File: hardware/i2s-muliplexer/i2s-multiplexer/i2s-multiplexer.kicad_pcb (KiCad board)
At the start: 2 copper layers, 64.5 x 63.5 mm, 35 parts, among them J1 Conn_01x05, J2 Conn_01x05, J3 Conn_01x05, J4 Conn_01x05, J5 Conn_01x05, J6 Conn_01x05, J7 Conn_01x07, J8 Conn_01x05, U1 74HC244, U2 74HC244, U3 74HC244, U4 74HC126, U5 74LS138

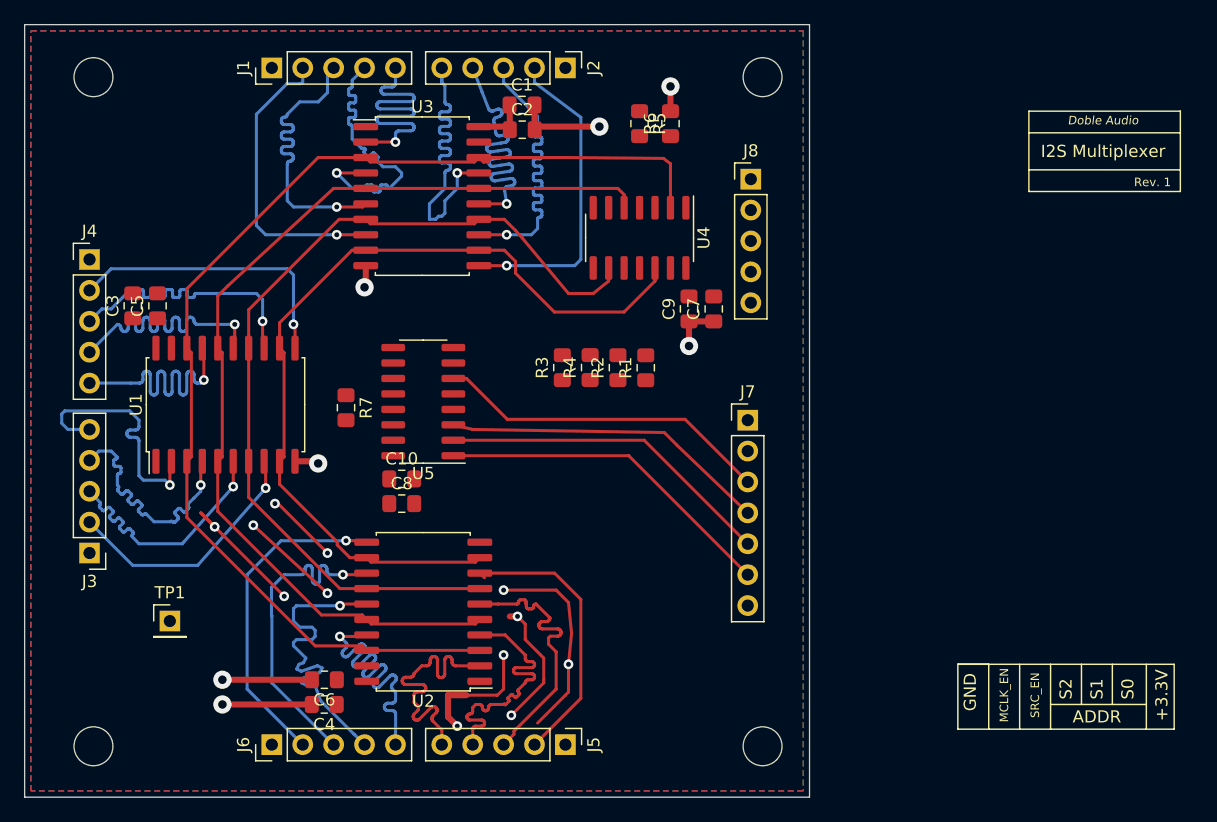
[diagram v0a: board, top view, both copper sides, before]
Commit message: Updated to KiCad 6
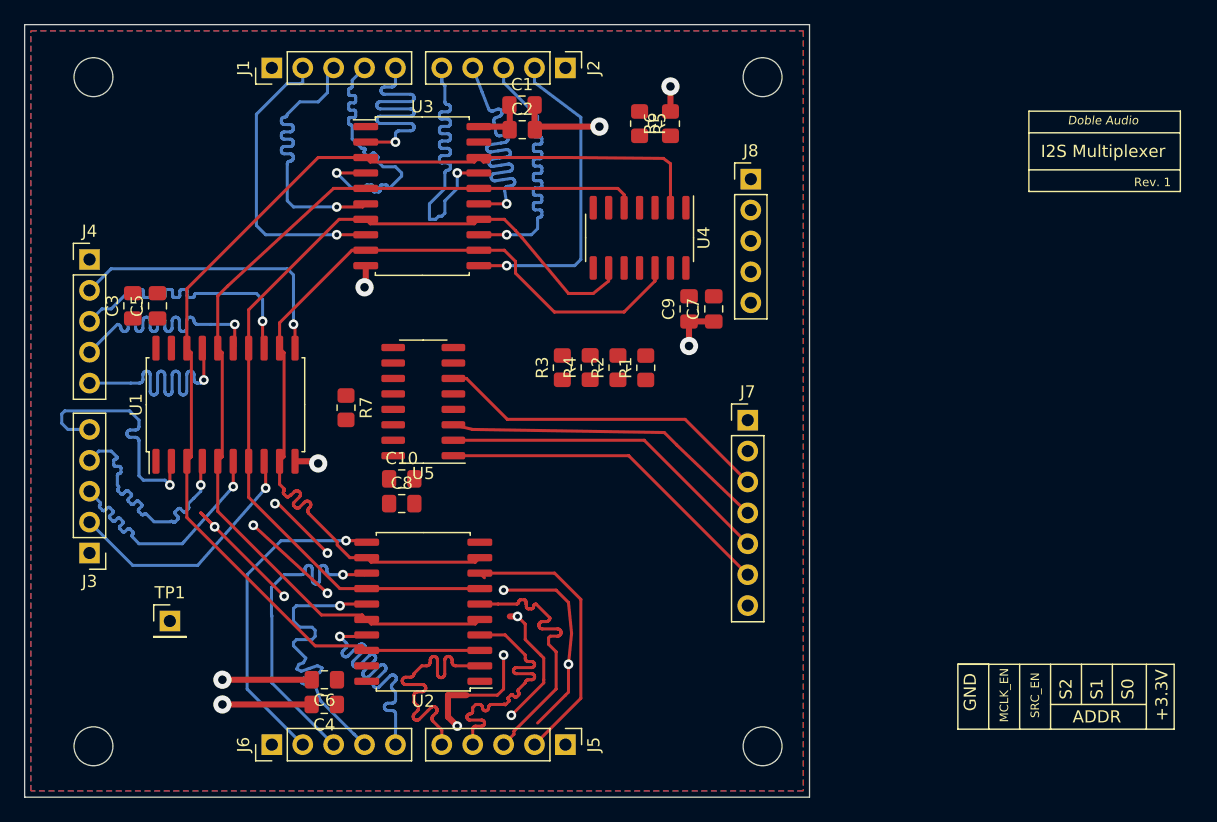
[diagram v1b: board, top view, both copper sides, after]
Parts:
- C1, C10, C2, C3, C4, C5, C6, C7, C8, C9: footprint Capacitor_SMD:C_0805_2012Metric_Pad1.15x1.40mm_HandSolder -> Capacitor_SMD:C_0805_2012Metric_Pad1.18x1.45mm_HandSolder
- R1, R2, R3, R4, R5, R6, R7: footprint Resistor_SMD:R_0805_2012Metric_Pad1.15x1.40mm_HandSolder -> Resistor_SMD:R_0805_2012Metric_Pad1.20x1.40mm_HandSolder
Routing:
- net /MCLK: track 71.1 -> 74.4 mm
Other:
- net class Default removed
- net class Power removed
